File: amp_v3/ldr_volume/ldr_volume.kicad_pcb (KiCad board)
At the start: 2 copper layers, 316.9 x 199.6 mm, 163 parts, among them J1 PWR1, J10 5v_in, J11 CTRL, J12 I2C_R, J13 A_IN, J14 A_OUT, J15 ADS1115, J16 MUTE_OUT, J17 MUTE, J18 UART, J19 MUTE, J2 PWR2, J20 CTRL, J21 CTRL, J22 PWR_IN, J23 I2C_L, J24 I2C_R, J26 TFT, J27 PWR_BTN, J28 PWR_BTN_LED, J29 PWR_IN, J3 PWR3, J30 I2C, J31 BTN_VOL, J32 BTN_MENU, J33 ALPS, J34 PWR_RLY, J35 BTN_EXT1, J36 BTN_EXT2, J38 IR, J39 MUTE, J4 PWR4, J40 UART, J41 IR_SENSOR, J42 S_AIN_L, J43 S_AIN_R, J5 PWR3, J6 PWR4, J7 Conn_01x03_Pin, J8 5V_IN, J9 5V_IN, K1 G5V-2, Q1 BC557, Q10 2N7000, Q11 BC547, Q12 BC547, Q2 BC557, Q3 BC547, Q4 BC547, Q5 BC557, Q6 BC557, Q7 BC547, Q8 BC547, Q9 2N7000, SW1 SW_LT, SW2 SW_RT, SW3 SW_UP, SW4 SW_DN, SW5 SW_PWR, U1 IRM-10-5, U2 NSL-32-SR3-Rseries, U3 MCP1700x-330xxTO, U4 NSL-32-SR3-Rshunt, U5 4N25, U6 TSOP312xx

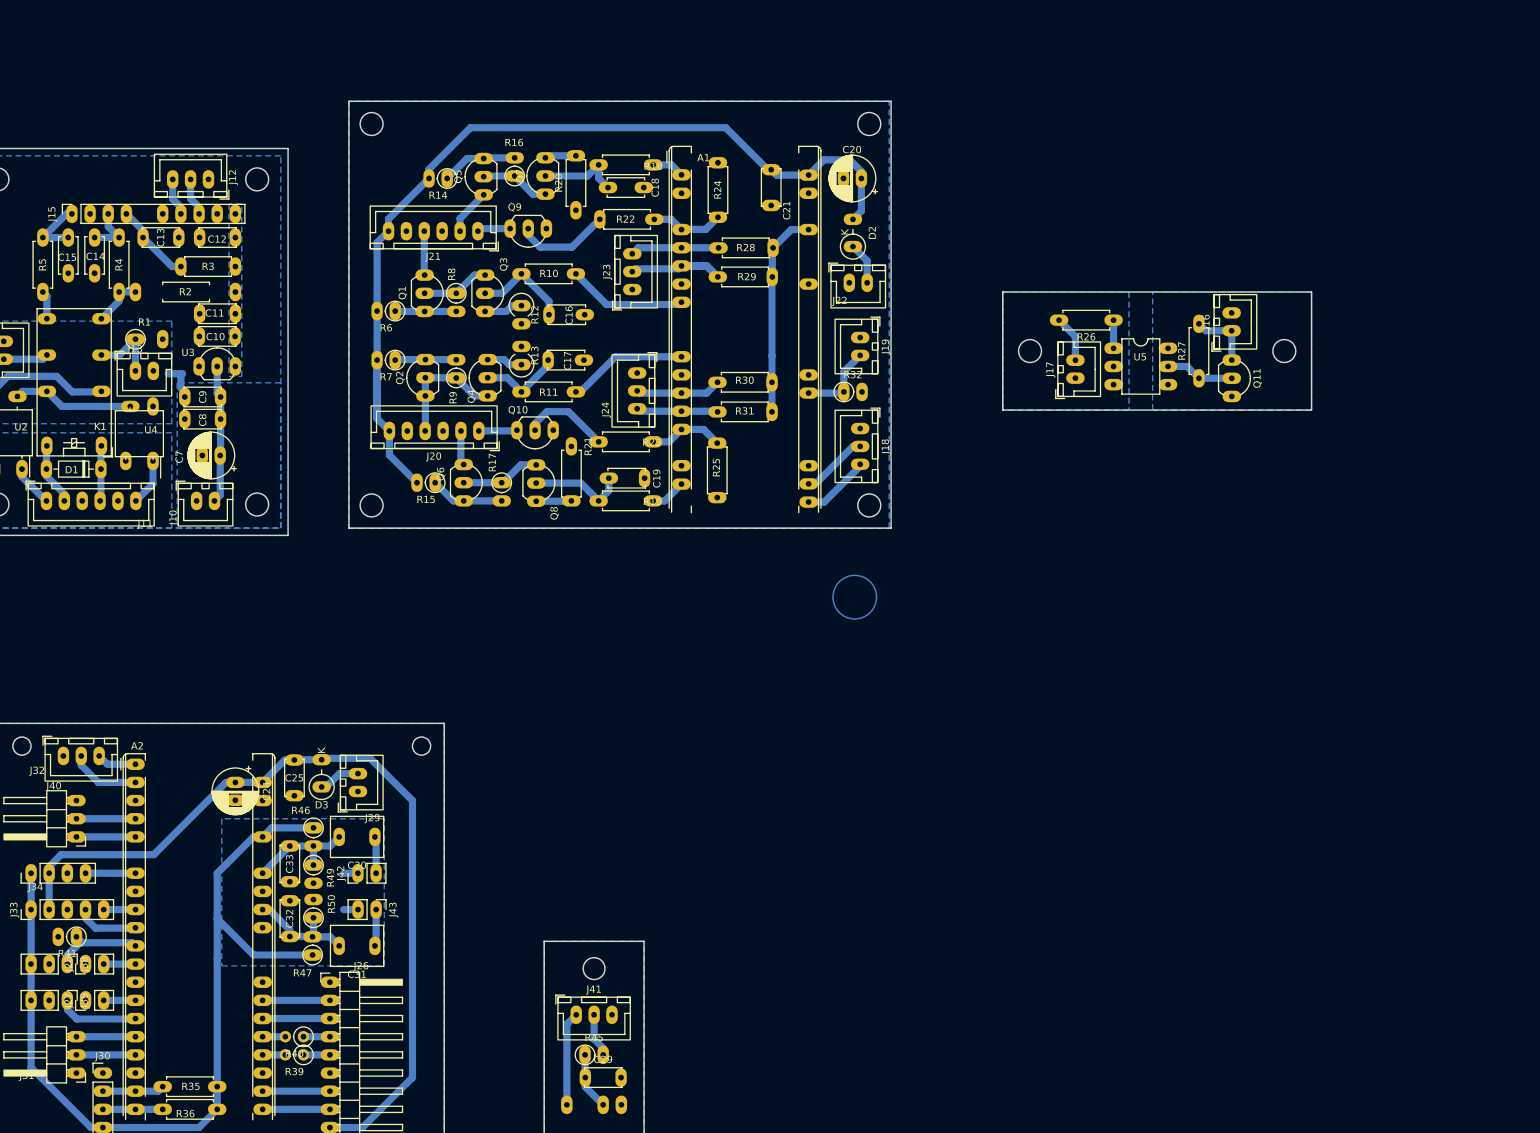
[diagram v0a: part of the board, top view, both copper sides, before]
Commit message: updates v1b
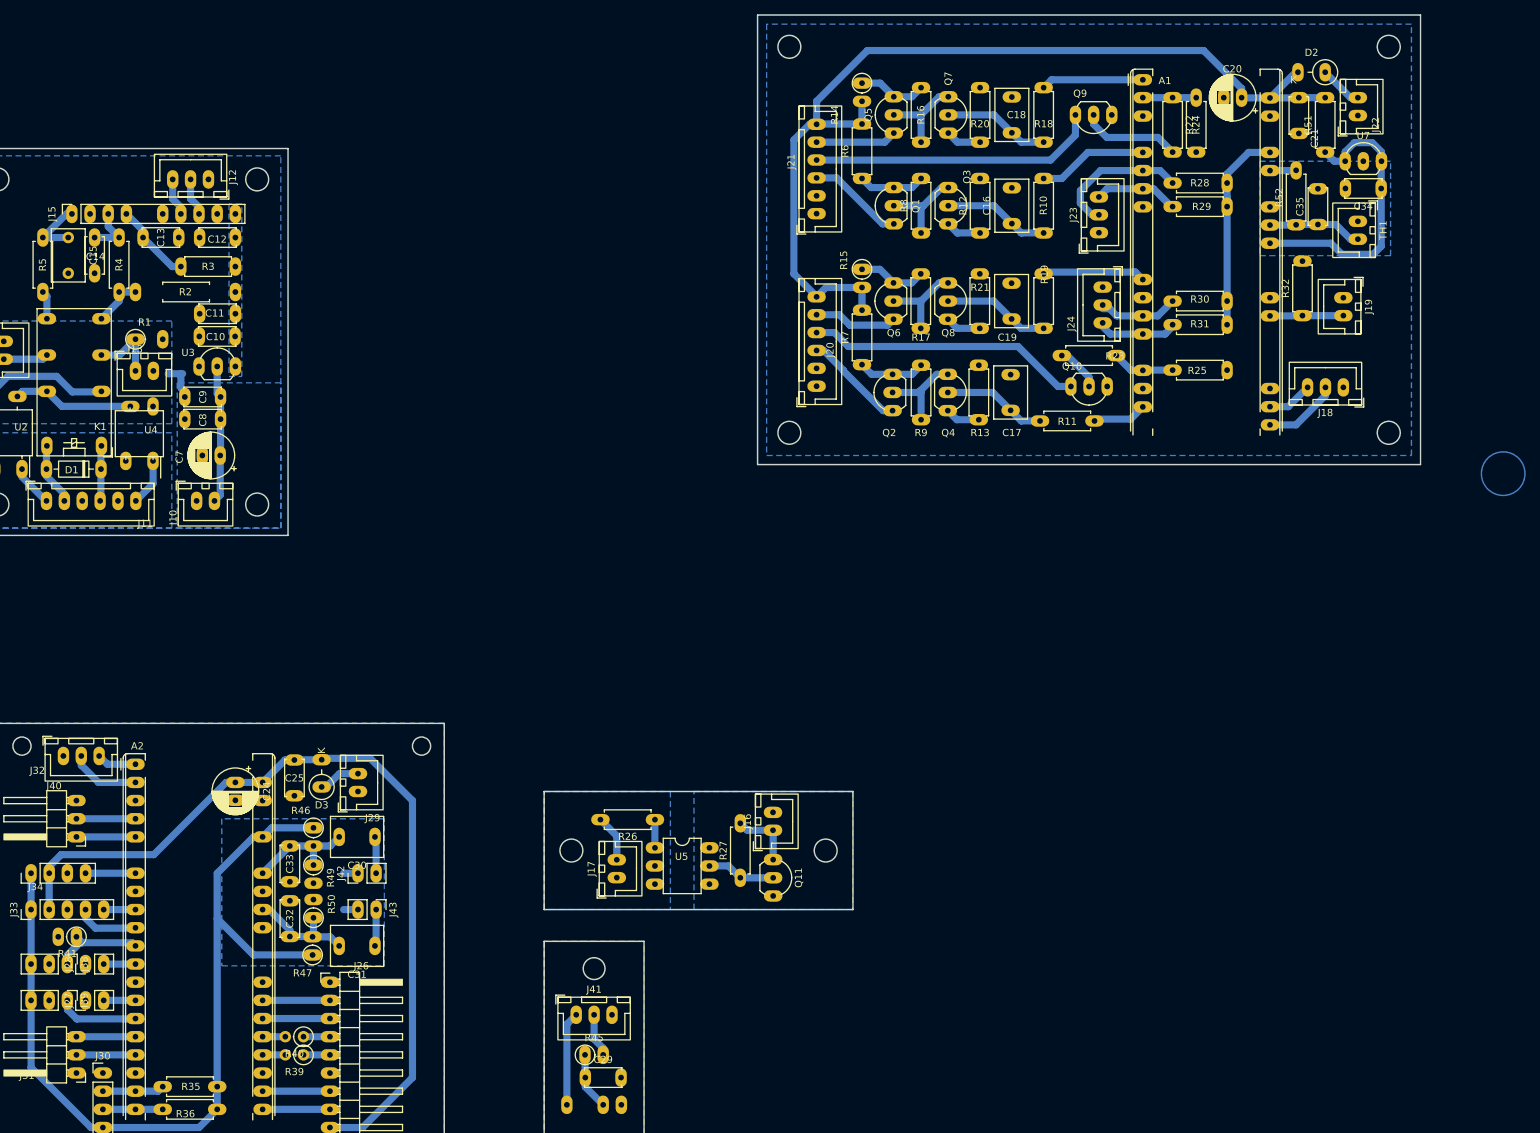
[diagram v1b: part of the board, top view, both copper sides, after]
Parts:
- added C34: 100nF, Capacitor_THT:C_Disc_D5.0mm_W2.5mm_P5.00mm, F.Cu at (219.8, -158.7)
- added C35: 100nF, Capacitor_THT:C_Disc_D5.0mm_W2.5mm_P5.00mm, F.Cu at (211.0, -153.6)
- added R51: 2.2K, Resistor_THT:R_Axial_DIN0207_L6.3mm_D2.5mm_P7.62mm_Horizontal, F.Cu at (212.0, -163.7)
- added R52: 100K, Resistor_THT:R_Axial_DIN0207_L6.3mm_D2.5mm_P7.62mm_Horizontal, F.Cu at (207.9, -153.6)
- added TH1: B3950, Connector_JST:JST_XH_B2B-XH-A_1x02_P2.50mm_Vertical, F.Cu at (216.6, -154.1)
- added U7: TL431LP, Package_TO_SOT_THT:TO-92_Inline_Wide, F.Cu at (214.8, -162.5)
- C15, C16, C17, C18, C19: footprint Capacitor_THT:C_Disc_D5.0mm_W2.5mm_P5.00mm -> Capacitor_THT:C_Rect_L7.2mm_W4.5mm_P5.00mm_FKS2_FKP2_MKS2_MKP2
- R12, R13: footprint Resistor_THT:R_Axial_DIN0309_L9.0mm_D3.2mm_P2.54mm_Vertical -> Resistor_THT:R_Axial_DIN0207_L6.3mm_D2.5mm_P7.62mm_Horizontal
- R16, R17, R8, R9: value 1M -> 100K; footprint Resistor_THT:R_Axial_DIN0207_L6.3mm_D2.5mm_P2.54mm_Vertical -> Resistor_THT:R_Axial_DIN0207_L6.3mm_D2.5mm_P7.62mm_Horizontal
- R32, R6, R7: footprint Resistor_THT:R_Axial_DIN0207_L6.3mm_D2.5mm_P2.54mm_Vertical -> Resistor_THT:R_Axial_DIN0207_L6.3mm_D2.5mm_P7.62mm_Horizontal
- moved R27 94.8 mm to (130.2, -62.3)
- moved J16 94.8 mm to (134.8, -68.9)
- moved J17 94.8 mm to (112.9, -62.3)
- moved Q11 94.8 mm to (134.8, -64.8)
- moved R26 94.8 mm to (118.3, -70.4)
- moved U5 94.8 mm to (118.3, -66.5)
- moved Q9 80.6 mm to (182.2, -168.9)
- moved Q10 77.7 mm to (181.5, -131.0)
- moved J22 74.9 mm to (216.6, -168.9), turned to 90 degrees
- moved C21 74.5 mm to (208.3, -171.4)
- moved R22 74.4 mm to (190.7, -171.4), turned to -90 degrees
- moved R10 73.2 mm to (172.6, -152.4), turned to 90 degrees
- moved R11 72.6 mm to (172.1, -126.2)
- moved R24 68.9 mm to (194.0, -171.4), turned to -90 degrees
- moved R6 67.9 mm to (147.2, -160.1), turned to 90 degrees
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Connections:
- A1 pad 12: /LDR Driver/PWM_SHUNT_R -> /LDR Driver/PWM_SER_R
- A1 pad 19: /LDR Driver/PWM_SER_R -> /LDR Driver/PWM_SHUNT_R
- A1 pad 2: /LDR Driver/PWM_SER_L -> /LDR Driver/COIL_CTRL_L
- A1 pad 33: GNDD -> /LDR Driver/AGND_PICO
- A1 pad 5: /LDR Driver/COIL_CTRL_L -> /LDR Driver/PWM_SHUNT_L
- J20 pad 1: /LDR Driver/COIL_R -> GNDD
- J20 pad 2: /LDR Driver/SERIAL_R -> GNDD
- J20 pad 3: GNDD -> /LDR Driver/SHUNT_R
- J20 pad 4: /LDR Driver/SHUNT_R -> /LDR Driver/COIL_R
- J20 pad 5: GNDD -> /LDR Driver/SERIAL_R
- J21 pad 1: /LDR Driver/COIL_L -> GNDD
- J21 pad 2: /LDR Driver/SERIAL_L -> GNDD
- J21 pad 3: GNDD -> /LDR Driver/SHUNT_L
- J21 pad 4: /LDR Driver/SHUNT_L -> /LDR Driver/COIL_L
- J21 pad 5: GNDD -> /LDR Driver/SERIAL_L
- J23 pad 2: /LDR Driver/SCL_L -> /LDR Driver/SDA_L
- J23 pad 3: /LDR Driver/SDA_L -> /LDR Driver/SCL_L
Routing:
- net /LDR Driver/ADC_TL431REF: track 0.00 -> 40.6 mm
- net /LDR Driver/COIL_L: track 4.65 -> 40.5 mm
- net /LDR Driver/COIL_R: track 5.37 -> 38.7 mm
- net /LDR Driver/ADC_NTC: track 0.00 -> 13.1 mm
- net Net-(Q2-B): track 0.00 -> 12.9 mm
- net /LDR Driver/PWM_SER_L: track 4.54 -> 14.3 mm
- net /LDR Driver/PWM_SER_R: track 4.94 -> 14.4 mm
- net /LDR Driver/PWM_SHUNT_R: track 16.2 -> 7.47 mm
- net /LDR Driver/SDA_L: track 12.4 -> 19.8 mm
- net /LDR Driver/SHUNT_L: track 6.10 -> 13.5 mm
- net /LDR Driver/SCL_L: track 18.8 -> 11.8 mm
- net Net-(Q10-G): track 13.2 -> 6.36 mm
- net /LDR Driver/SERIAL_R: track 5.40 -> 11.7 mm
- net /LDR Driver/SERIAL_L: track 6.45 -> 11.3 mm
- net /LDR Driver/ADC_VREF: track 0.00 -> 3.62 mm
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- added copper zone on B.Cu, net /LDR Driver/AGND_PICO
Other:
- board size 316.9 x 199.6 mm -> 332.1 x 201.9 mm

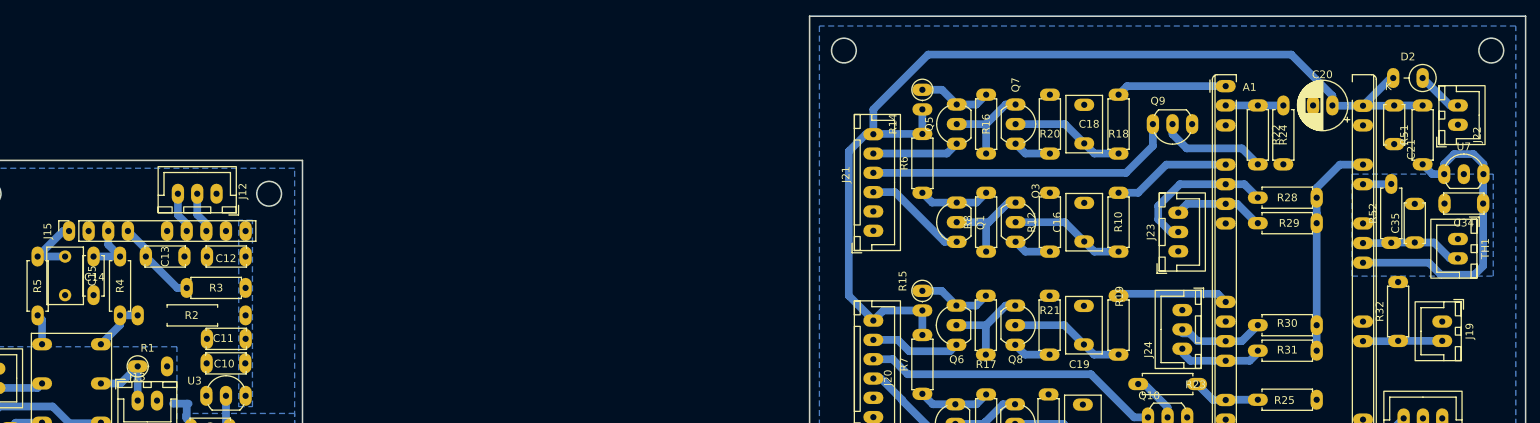
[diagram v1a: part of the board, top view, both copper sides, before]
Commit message: updates
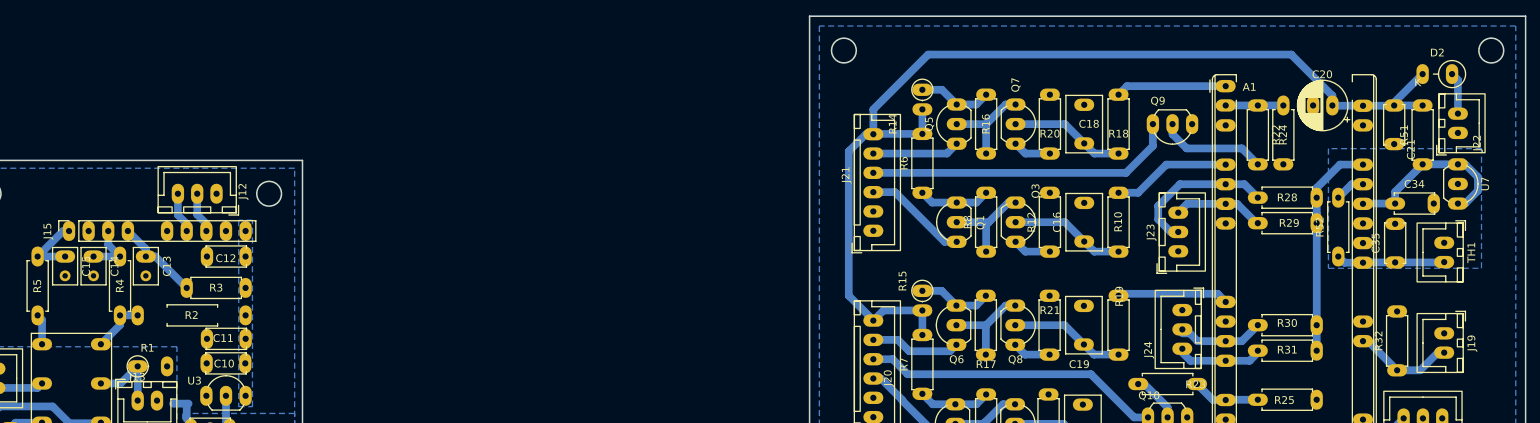
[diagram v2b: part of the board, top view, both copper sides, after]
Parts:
- C13, C14: footprint Capacitor_THT:C_Disc_D5.0mm_W2.5mm_P5.00mm -> Capacitor_THT:C_Rect_L4.6mm_W3.0mm_P2.50mm_MKS02_FKP02
- C15: footprint Capacitor_THT:C_Rect_L7.2mm_W4.5mm_P5.00mm_FKS2_FKP2_MKS2_MKP2 -> Capacitor_THT:C_Rect_L4.6mm_W3.0mm_P2.50mm_MKS02_FKP02
- moved C34 11.4 mm to (208.4, -158.7), turned to 0 degrees
- moved R52 7.08 mm to (201.1, -151.8)
- moved D2 3.84 mm to (212.0, -175.4)
- moved R32 3.81 mm to (208.7, -137.1)
- moved C35 3.62 mm to (208.4, -151.0)
- moved U7 2.18 mm to (216.6, -163.7), turned to -90 degrees
- moved TH1 1.84 mm to (214.8, -153.6)
- moved J19 1.55 mm to (214.8, -141.9)
- moved J22 1.06 mm to (216.6, -167.8)
- turned C13 to -90 degrees
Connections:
- A1 pad 31: /LDR Driver/ADC_TL431REF -> /LDR Driver/ADC_NTC
- A1 pad 32: /LDR Driver/ADC_NTC -> /LDR Driver/AGND_PICO
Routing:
- net /LDR Driver/ADC_TL431REF: track 40.6 -> 23.6 mm
- net /LDR Driver/MUTE_CTRL: track 16.8 -> 18.8 mm
- net /LDR Driver/ADC_NTC: track 13.1 -> 14.1 mm
- net /LDR Driver/5V_board1: track 6.04 -> 5.44 mm
